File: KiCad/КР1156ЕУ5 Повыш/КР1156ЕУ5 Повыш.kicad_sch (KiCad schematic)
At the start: 10 parts, among them U1 КР1156ЕУ5

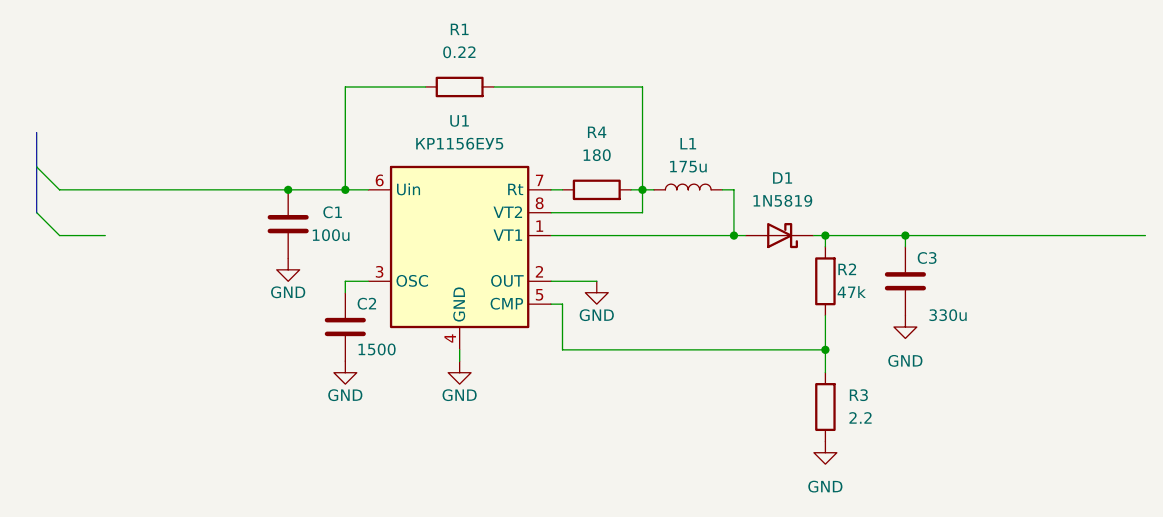
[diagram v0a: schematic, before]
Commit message: KF
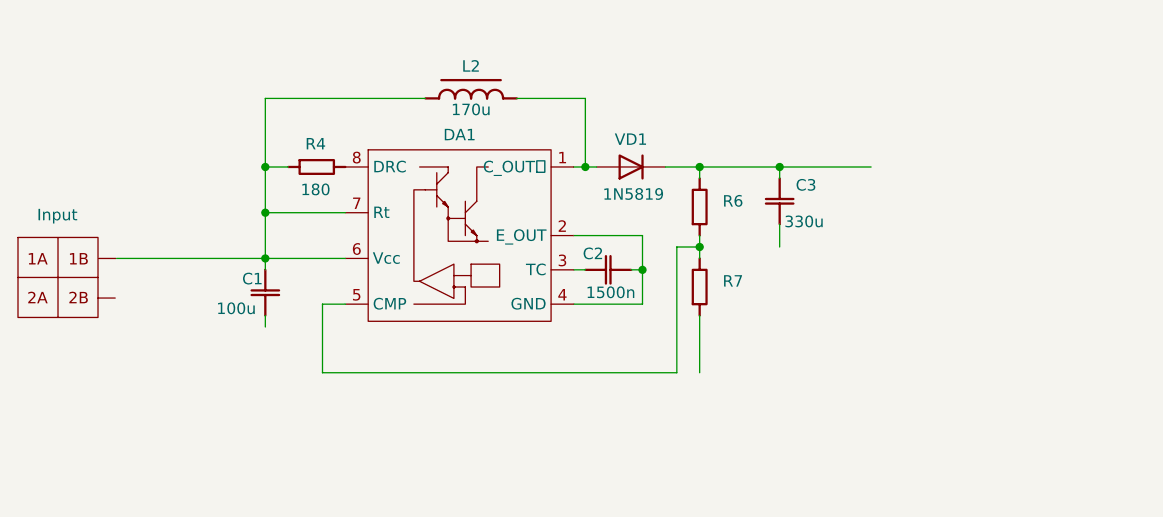
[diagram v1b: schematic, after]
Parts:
- removed C1: 100u, symbol Device:C
- removed C2: 1500, symbol Device:C
- removed C3: 330u, symbol Device:C
- removed L1: 175u, symbol Device:L
- removed R1: 0.22, symbol Device:R
- removed R2: 47k, symbol Device:R
- removed R3: 2.2, symbol Device:R
- removed R4: 180, symbol Device:R
- removed U1: КР1156ЕУ5, Package_SO:SOIC-8_3.9x4.9mm_P1.27mm, symbol work:MC33063AD
- added DА1: ~, symbol for work:КР1156ЕУ5
- added Input: ~, symbol for work:terminal_block_input
- added L2: 170u, symbol for work:Inductor
- added R4: 180, symbol for work:Resistor
- added R6, R7: ~, symbol for work:Resistor
- added С1: 100u, symbol for work:Capacitor
- added С2: 1500n, symbol for work:Capacitor
- added С3: 330u, symbol for work:Capacitor
- renumbered D1 to VD1
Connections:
- net at VD1.1 (K): now also R6., С3.
- net at VD1.2 (A): now also DА1.1 (C_OUT ), L2.
- new net: DА1.2 (E_OUT), DА1.4 (GND), С2.
- new net: DА1.3 (TC), С2.
- new net: DА1.5 (CMP), R6., R7.
- new net: DА1.6 (Vcc), DА1.7 (Rt), L2., R4., С1.
- new net: DА1.8 (DRC), R4.
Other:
- moved on the sheet: VD1
